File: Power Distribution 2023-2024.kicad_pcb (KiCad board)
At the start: 2 copper layers, 53.3 x 55.2 mm, 29 parts, among them J1 TEL_OUT, J2 STEER_OUT, J3 SAFE_OUT, J4 12V_IN, J5 L_KILL, J6 R_KILL, J7 SAFE_KILL

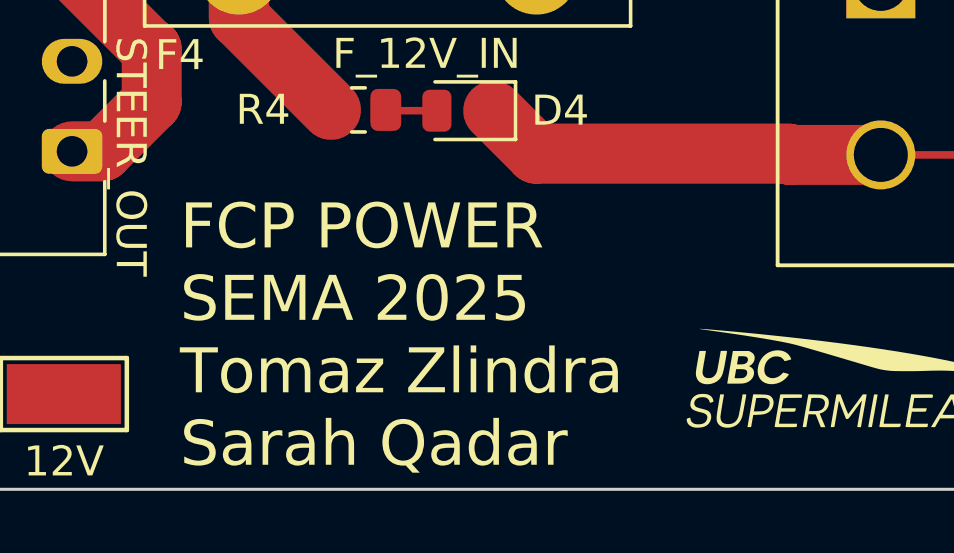
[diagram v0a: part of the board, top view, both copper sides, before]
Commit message: December 2nd, 2023
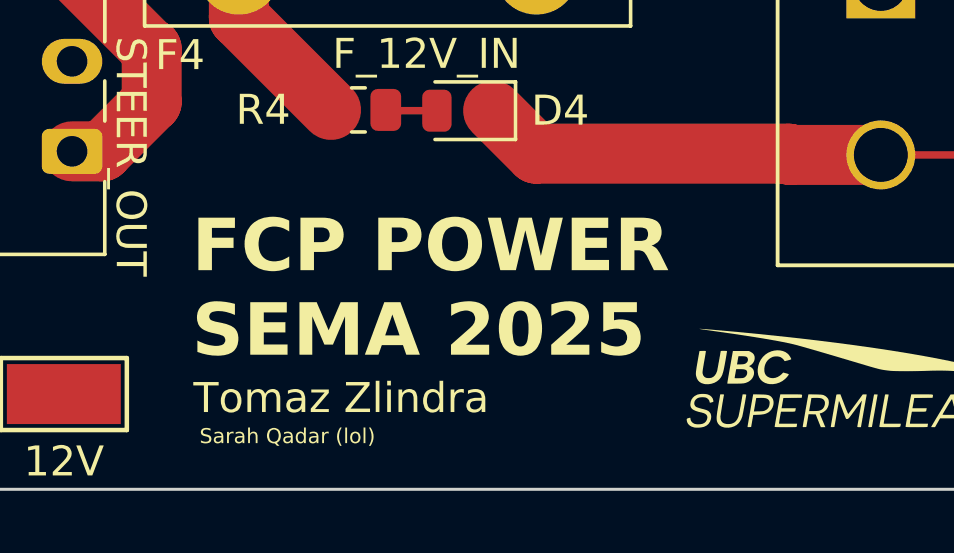
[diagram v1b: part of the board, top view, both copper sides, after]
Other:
- board text added: "FCP POWER SEMA 2025"
- board text added: "Sarah Qadar (lol)"
- board text added: "Tomaz Zlindra"
- board text removed: "FCP POWER SEMA 2025 Tomaz Zlindra Sarah Qadar"
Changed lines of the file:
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@@
   (gr_rect (start 213.36 97.79) (end 266.7 153.035)
     (stroke (width 0.1) (type default)) (fill none) (layer "Edge.Cuts"))
-  (gr_text "FCP POWER\nSEMA 2025\nTomaz Zlindra\nSarah Qadar" (at 226.06 152.4) (layer "F.SilkS")
-    (effects (font (size 1.5 1.5) (thickness 0.225)) (justify left bottom))
+  (gr_text "FCP POWER\nSEMA 2025\n" (at 226.452733 148.762235) (layer "F.SilkS")
+    (effects (font (size 1.75 1.75) (thickness 0.3) bold) (justify left bottom))
   )
   (gr_text "F_STEER" (at 219.772096 113.856974) (layer "F.SilkS")
@@
     (effects (font (size 1 1) (thickness 0.15)) (justify left bottom))
   )
+  (gr_text "Tomaz Zlindra" (at 226.50624 150.581461) (layer "F.SilkS")
+    (effects (font (size 1 1) (thickness 0.15)) (justify left bottom))
+  )
+  (gr_text "Sarah Qadar (lol)" (at 226.709884 151.557309) (layer "F.SilkS")
+    (effects (font (size 0.5 0.5) (thickness 0.1)) (justify left bottom))
+  )
   (gr_text "F_KILL" (at 228.569116 113.848962) (layer "F.SilkS")
